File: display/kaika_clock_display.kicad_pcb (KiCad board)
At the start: 2 copper layers, 128 x 32 mm, 21 parts, among them J1 Conn_01x05, U1 MAX7219, U2 MAX7219, U3 MAX7219, U4 MAX7219, U5 LED-MATRIX-1088AS, U6 LED-MATRIX-1088AS, U7 LED-MATRIX-1088AS, U8 LED-MATRIX-1088AS

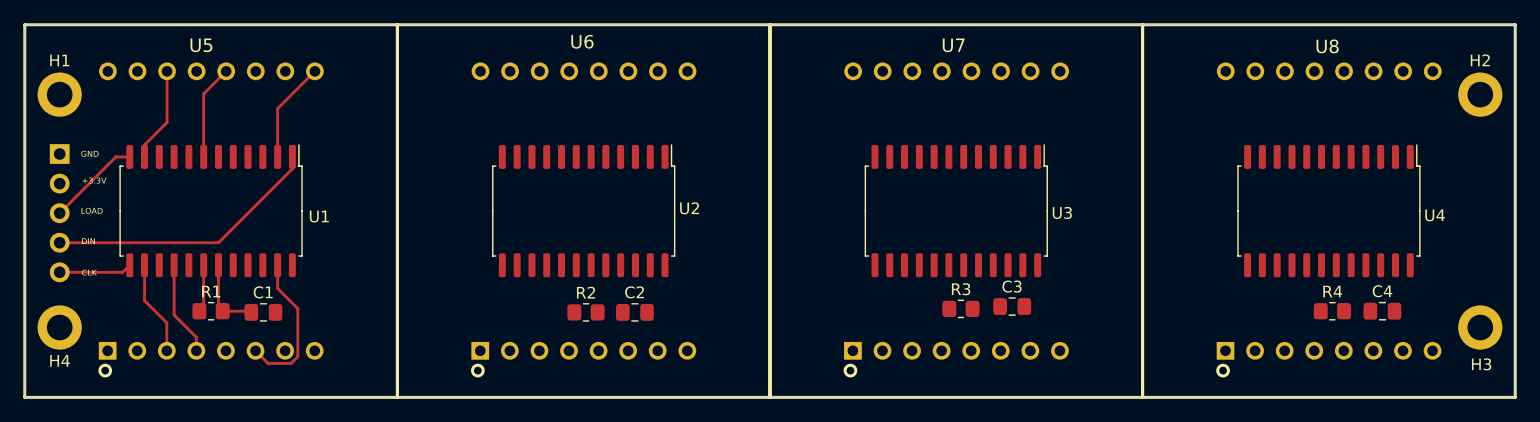
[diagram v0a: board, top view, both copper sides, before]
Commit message: finish display board draw.
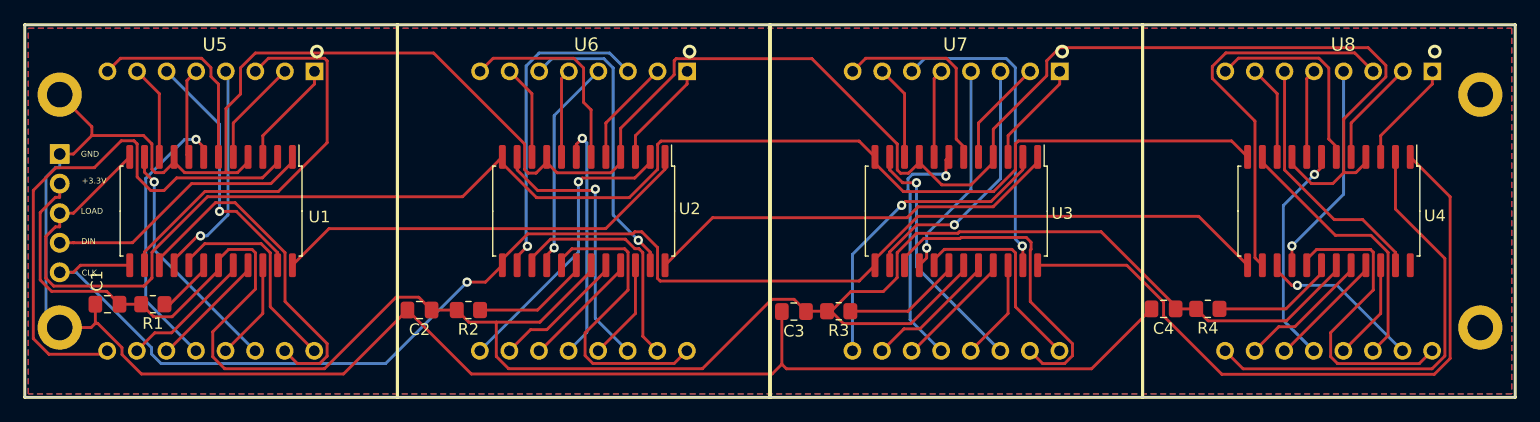
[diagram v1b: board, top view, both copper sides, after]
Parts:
- moved C4 18.8 mm to (197.8, 124.4), turned to 180 degrees
- moved C3 18.8 mm to (166.1, 124.6), turned to 180 degrees
- moved C2 18.5 mm to (133.9, 124.5), turned to 180 degrees
- moved C1 13.4 mm to (107.1, 124.0), turned to 180 degrees
- moved R4 10.7 mm to (201.6, 124.4), turned to 180 degrees
- moved R3 10.5 mm to (169.9, 124.6), turned to 180 degrees
- moved R2 10.1 mm to (138.1, 124.5), turned to 180 degrees
- moved R1 5.04 mm to (111.0, 124.0), turned to 180 degrees
- turned U5 to 180 degrees
- turned U6 to 180 degrees
- turned U7 to 180 degrees
- turned U8 to 180 degrees
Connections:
- H1 pad 1: (no net) -> GND
- H4 pad 1: (no net) -> GND
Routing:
- net GND: track 0.00 -> 307.9 mm
- net +3V3: track 6.61 -> 183.4 mm
- net LOAD: track 8.02 -> 134.4 mm
- net CLK: track 6.27 -> 124.5 mm, vias 0 -> 1
- net Net-(U3-Pad24): track 0.00 -> 59.3 mm
- net 4_DIG_0: track 0.00 -> 38.8 mm
- net 1_DIG_0: track 8.68 -> 47.4 mm
- net Net-(U1-Pad24): track 0.00 -> 36.5 mm
- net Net-(U2-Pad24): track 0.00 -> 36.1 mm
- net 4_SEG_A: track 0.00 -> 33.8 mm
- net 1_SEG_F: track 0.00 -> 29.9 mm
- net 3_SEG_F: track 0.00 -> 28.1 mm
- net 2_SEG_A: track 0.00 -> 27.4 mm, vias 0 -> 1
- net 3_DIG_0: track 0.00 -> 27.0 mm, vias 0 -> 1
- net 3_SEG_D: track 0.00 -> 26.9 mm, vias 0 -> 1
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- added copper zone on B.Cu, net GND
- added copper zone on F.Cu, net GND
